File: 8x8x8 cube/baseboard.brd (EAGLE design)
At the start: 156 x 156 mm, 100 parts, among them IC1 LM321MF, J1 CONNECTOR-HEADER-2X2P2X2P-2.5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, J10 CONNECTOR-HEADER-2X2P2X2P-2.5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, J11 CONNECTOR-HEADER-2X2P2X2P-2.5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, J12 CONNECTOR-HEADER-2X2P2X2P-2.5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, J13 CONNECTOR-HEADER-2X2P2X2P-2.5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, J14 CONNECTOR-HEADER-2X2P2X2P-2.5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, J15 CONNECTOR-HEADER-2X2P2X2P-2.5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, J16 CONNECTOR-HEADER-2X2P2X2P-2.5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, J17 CONNECTOR-HEADER-2X2P2X2P-2.5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, J18 CONNECTOR-HEADER-2X2P2X2P-2.5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, J19 CONNECTOR-HEADER-2X2P2X2P-2.5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, J2 CONNECTOR-HEADER-2X2P2X2P-2.5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, J20 CONNECTOR-HEADER-2X2P2X2P-2.5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, J21 CONNECTOR-HEADER-2X2P2X2P-2.5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, J22 CONNECTOR-HEADER-2X2P2X2P-2.5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, J23 CONNECTOR-HEADER-2X2P2X2P-2.5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, J24 CONNECTOR-HEADER-2X2P2X2P-2.5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, J25 CONNECTOR-HEADER-2X2P2X2P-2.5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, J26 CONNECTOR-HEADER-2X2P2X2P-2.5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, J27 CONNECTOR-HEADER-2X2P2X2P-2.5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, J28 CONNECTOR-HEADER-2X2P2X2P-2.5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, J29 CONNECTOR-HEADER-2X2P2X2P-2.5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, J3 CONNECTOR-HEADER-2X2P2X2P-2.5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, J30 CONNECTOR-HEADER-2X2P2X2P-2.5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, J31 CONNECTOR-HEADER-2X2P2X2P-2.5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, J32 CONNECTOR-HEADER-2X2P2X2P-2.5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, J33 CONNECTOR-HEADER-2X2P2X2P-2.5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, J34 CONNECTOR-HEADER-2X2P2X2P-2.5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, J35 CONNECTOR-HEADER-2X2P2X2P-2.5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, J36 CONNECTOR-HEADER-2X2P2X2P-2.5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, J37 CONNECTOR-HEADER-2X2P2X2P-2.5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, J38 CONNECTOR-HEADER-2X2P2X2P-2.5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, J39 CONNECTOR-HEADER-2X2P2X2P-2.5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, J4 CONNECTOR-HEADER-2X2P2X2P-2.5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, J40 CONNECTOR-HEADER-2X2P2X2P-2.5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, J41 CONNECTOR-HEADER-2X2P2X2P-2.5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, J42 CONNECTOR-HEADER-2X2P2X2P-2.5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, J43 CONNECTOR-HEADER-2X2P2X2P-2.5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, J44 CONNECTOR-HEADER-2X2P2X2P-2.5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, J45 CONNECTOR-HEADER-2X2P2X2P-2.5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, J46 CONNECTOR-HEADER-2X2P2X2P-2.5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, J47 CONNECTOR-HEADER-2X2P2X2P-2.5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, J48 CONNECTOR-HEADER-2X2P2X2P-2.5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, J49 CONNECTOR-HEADER-2X2P2X2P-2.5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, J5 CONNECTOR-HEADER-2X2P2X2P-2.5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, J50 CONNECTOR-HEADER-2X2P2X2P-2.5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, J51 CONNECTOR-HEADER-2X2P2X2P-2.5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, J52 CONNECTOR-HEADER-2X2P2X2P-2.5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, J53 CONNECTOR-HEADER-2X2P2X2P-2.5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, J54 CONNECTOR-HEADER-2X2P2X2P-2.5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, J55 CONNECTOR-HEADER-2X2P2X2P-2.5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, J56 CONNECTOR-HEADER-2X2P2X2P-2.5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, J57 CONNECTOR-HEADER-2X2P2X2P-2.5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, J58 CONNECTOR-HEADER-2X2P2X2P-2.5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, J59 CONNECTOR-HEADER-2X2P2X2P-2.5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, J6 CONNECTOR-HEADER-2X2P2X2P-2.5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, J60 CONNECTOR-HEADER-2X2P2X2P-2.5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, J61 CONNECTOR-HEADER-2X2P2X2P-2.5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, J62 CONNECTOR-HEADER-2X2P2X2P-2.5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, J63 CONNECTOR-HEADER-2X2P2X2P-2.5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, J64 CONNECTOR-HEADER-2X2P2X2P-2.5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, J7 CONNECTOR-HEADER-2X2P2X2P-2.5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, J8 CONNECTOR-HEADER-2X2P2X2P-2.5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, J9 CONNECTOR-HEADER-2X2P2X2P-2.5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, Q3 MOSFET-N-044020001, U2 ADXL335

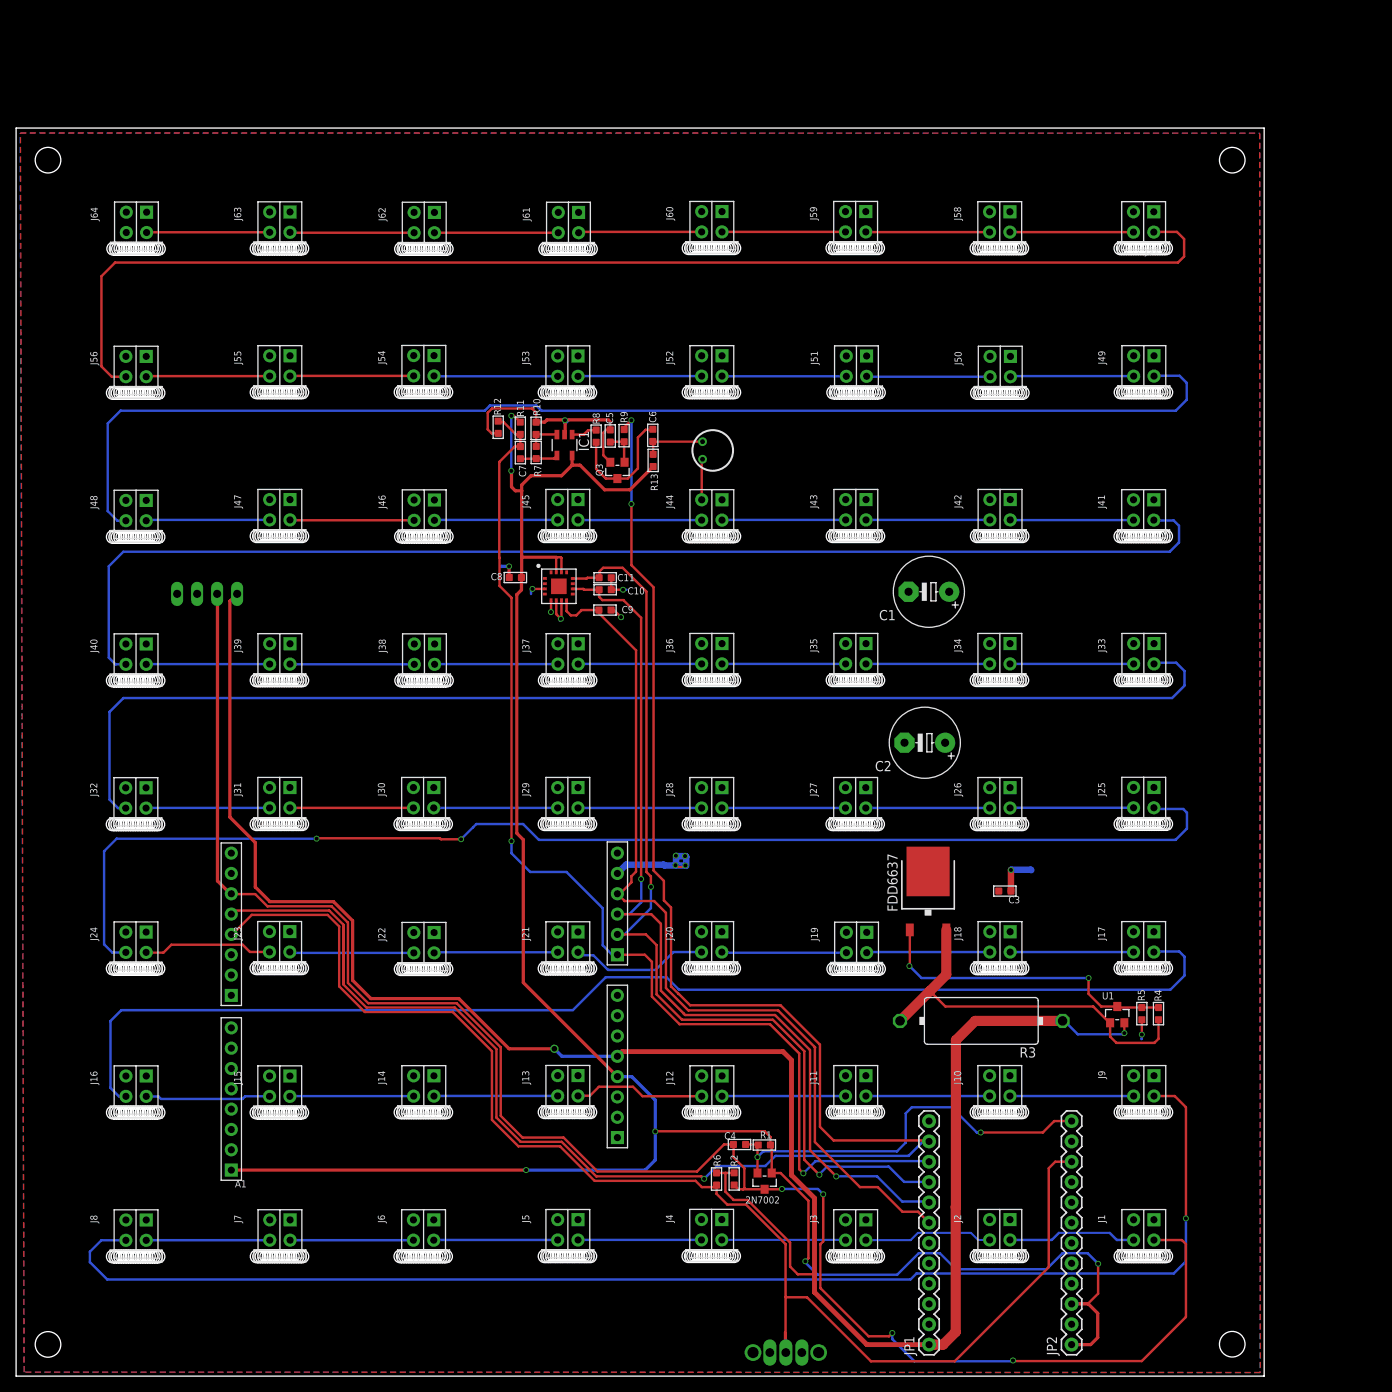
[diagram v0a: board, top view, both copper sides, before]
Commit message: updated to rev 7
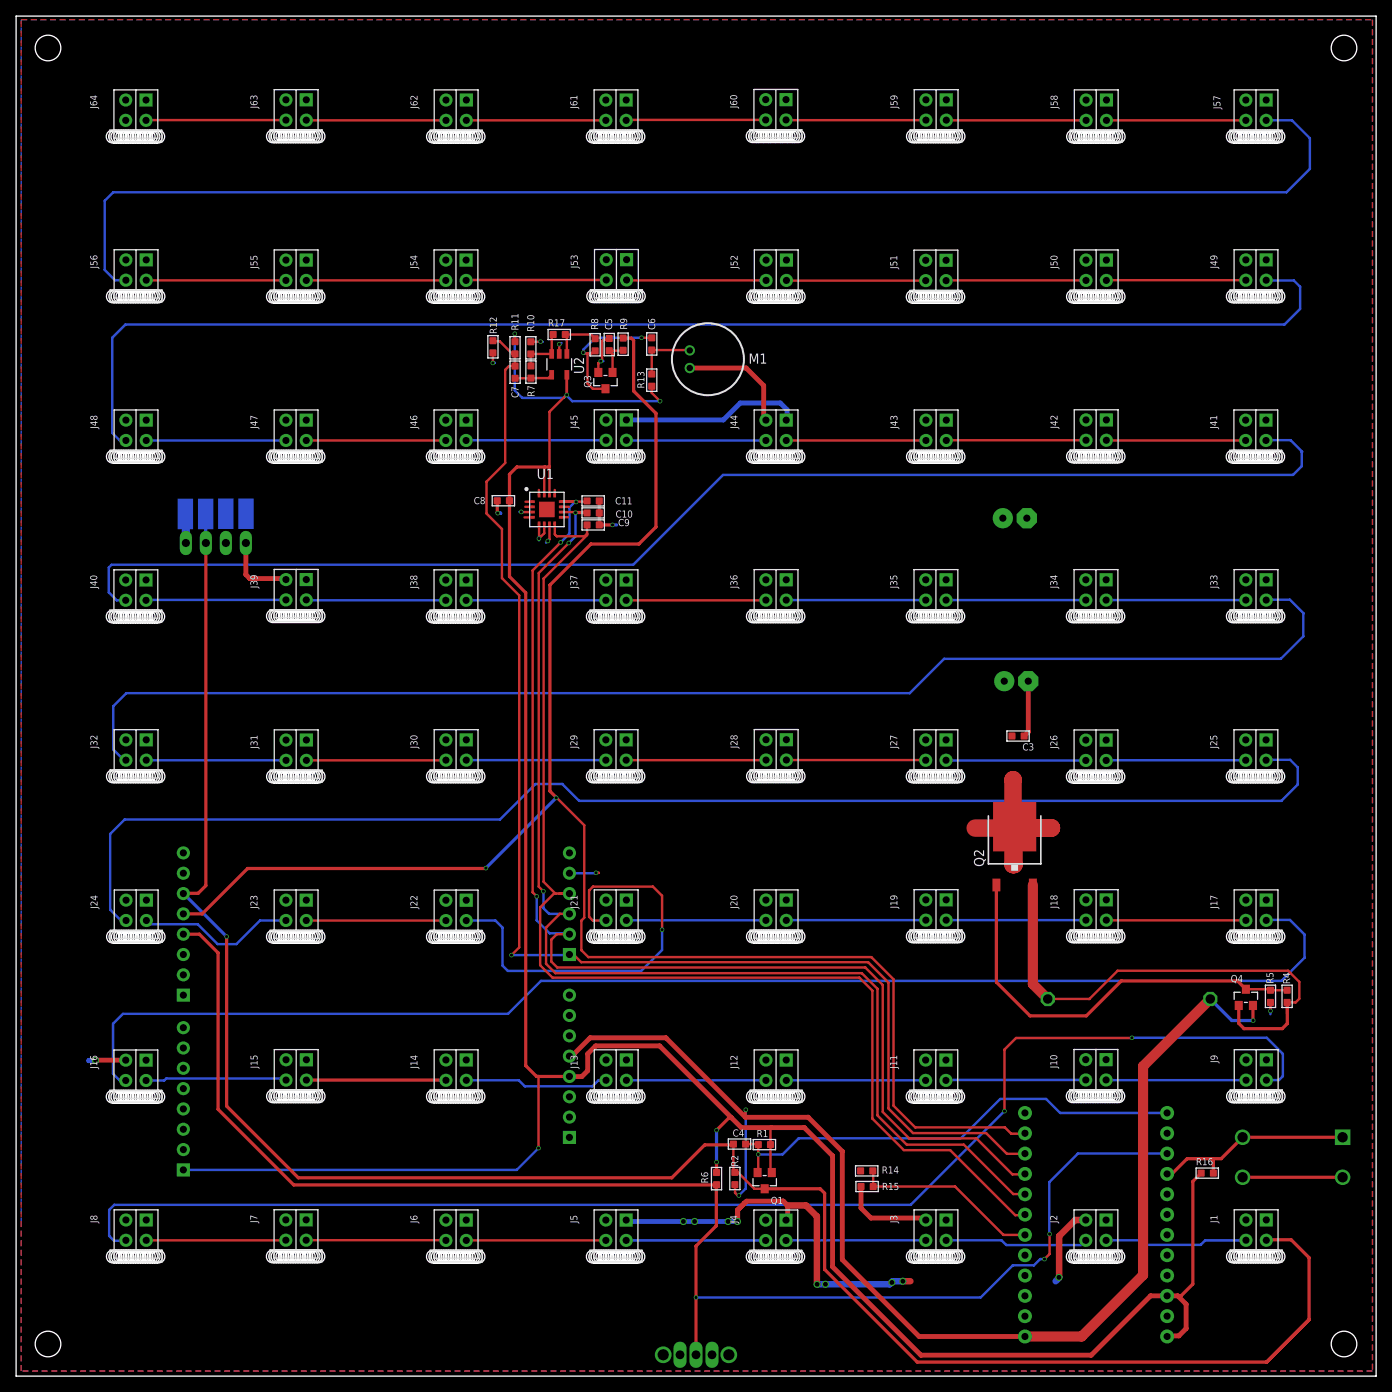
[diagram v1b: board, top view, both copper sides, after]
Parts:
- removed 2N7002: MOSFET-N-044020001, OPL Eagle Library:SOT23
- removed FDD6637: FDD4141TO252, transistor-fet:TO252
- removed IC1: LM321MF, linear:SOT23-5
- added BUTTON: BUTTON-4P4P-12X12X6H, OPL Eagle Library:4P-12X12X6H
- added GOLD_ORB_SM1: OSHWLOGO_GOLD_ORB_MED, NBitWonder:OSHW1
- added M1: MICROPHONE, OPL Eagle Library:MICROPHONE
- added Q1: 2N7002, OPL Eagle Library:SOT23
- added Q2: FDD6637, transistor-fet:TO252
- added Q4: SS8550, OPL Eagle Library:SOT23
- added R14, R15, R16: 10K, OPL Eagle Library:R0603
- added R17: 100K, OPL Eagle Library:R0603
- C1, C2: device OPL Eagle Library:CAPACITOR-E5-8.5 -> OPL Eagle Library:CAPACITOR-E3-8
- C4: value 100pF -> DNP
- Q3: value MOSFET-N-044020001 -> 2N7002
- R1, R6: value (none) -> 10K
- R13: value 100K -> 4.7K
- R7: value 2M -> DNP
- SV1: device con-amp-mt:S04P -> OPL Eagle Library:S04P
- U$1: value MICROPHONE -> L3D-LOGOL3DCUBE-LOGO-0.8X2.5; device OPL Eagle Library:MICROPHONE -> OPL Eagle Library:L3DCUBE-LOGO-0.8X2.5
- U1: value (none) -> ADXL335; device OPL Eagle Library:SOT23 -> OPL Eagle Library:ADXL335
- U2: value ADXL335 -> LM321MF; device OPL Eagle Library:ADXL335 -> linear:SOT23-5
- moved U1 95.2 mm to (66.3, 108.3)
- moved U$1 69.5 mm to (147.2, 148.4), flipped to the bottom
- moved U2 27.7 mm to (67.9, 126.5), turned to 180 degrees
- moved J57 19.8 mm to (155.0, 158.2)
- moved C3 19.5 mm to (125.2, 80.0)
- moved R3 18.7 mm to (139.1, 47.1), flipped to the bottom, turned to 0 degrees
- moved J58 18.5 mm to (135.0, 158.2)
- moved J49 18.4 mm to (155.0, 138.3)
- moved J59 17.2 mm to (115.0, 158.3)
- moved J41 17.2 mm to (155.0, 118.2)
- moved J50 17.0 mm to (135.0, 138.2)
- moved R4 16.2 mm to (158.9, 47.5)
- moved R5 16.2 mm to (156.8, 47.5)
- moved J33 16.1 mm to (155.0, 98.3)
- moved J60 16.1 mm to (95.0, 158.3)
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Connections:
- removed net D3: JP2.9
- new net MODE: BUTTON.P$1, BUTTON.P$4, JP2.9, R16.2
- new net N$71: JP1.6, R14.2, R15.1
- net +3V3: now also Q1.1, R16.1, R6.1, U1.VSS1, U1.VSS2, U2.5; no longer 2N7002.1, IC1.5, U2.VSS1, U2.VSS2
- net +5V: now also Q4.2; no longer R6.1, SV1.1, U1.2
- net D0: now also Q1.2; no longer 2N7002.2
- net DIN: now also Q1.3, SV1.P$2; no longer 2N7002.3
- net GND: now also BUTTON.P$2, BUTTON.P$3, M1.GND, R15.2, SV1.P$4, U1.COM1, U1.COM2, U1.COM3, U1.COM4, U2.2; no longer IC1.2, U$1.GND, U2.COM1, U2.COM2, U2.COM3, U2.COM4
- net N$32: now also U2.4; no longer IC1.4
- net N$65: now also Q2.2, Q4.1; no longer FDD6637.2, U1.1
- net N$66: now also R17.1, U2.3; no longer IC1.3
- net N$67: now also Q2.1, Q4.3; no longer FDD6637.1, U1.3
- net N$69: now also R17.2, U2.1; no longer IC1.1
- net N$72: now also M1.IN; no longer U$1.IN
- net V+: now also Q2.3, R14.1, SV1.1, SV1.P$1; no longer FDD6637.3, JP1.6
- net XOUT: now also U1.X; no longer U2.X
- net YOUT: now also U1.Y; no longer U2.Y
- net ZOUT: now also U1.Z; no longer U2.Z
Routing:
- net V+: track 13.5 -> 111.9 mm, vias 4 -> 9
- net +5V: track 253.3 -> 159.6 mm, vias 2 -> 3
- net +3V3: track 280.1 -> 336.1 mm
- net DIN: track 222.0 -> 262.0 mm, vias 4 -> 1
- net ZOUT: track 113.0 -> 150.8 mm
- net N$18: track 15.5 -> 53.1 mm, vias 0 -> 1
- net GND: track 59.7 -> 96.6 mm, vias 9 -> 12
- net YOUT: track 115.9 -> 149.1 mm, vias 2 -> 3
- net XOUT: track 121.0 -> 149.7 mm, vias 2 -> 3
- net MODE: track 0.00 -> 25.7 mm
- net SOUND: track 141.1 -> 166.8 mm, vias 2 -> 1
- net MICROPH: track 240.7 -> 216.7 mm, vias 3 -> 2
- net N$71: track 0.00 -> 23.5 mm
- net N$63: track 157.6 -> 174.3 mm
- net N$65: track 48.6 -> 65.2 mm
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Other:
- board size 156 x 156 mm -> 170 x 170 mm
- board text added: "Join WiFi"
- board text added: "November 2014"
- board text added: "Offline/Online"
- board text added: "Rev 1.0,"
- board text added: "www.L3Dcube.com"
- board text removed: "Offline/Online Switch"
- board text removed: "www.lytelab.com"
